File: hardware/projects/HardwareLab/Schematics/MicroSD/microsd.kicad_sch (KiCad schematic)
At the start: 3 parts, among them J1 Conn_01x03

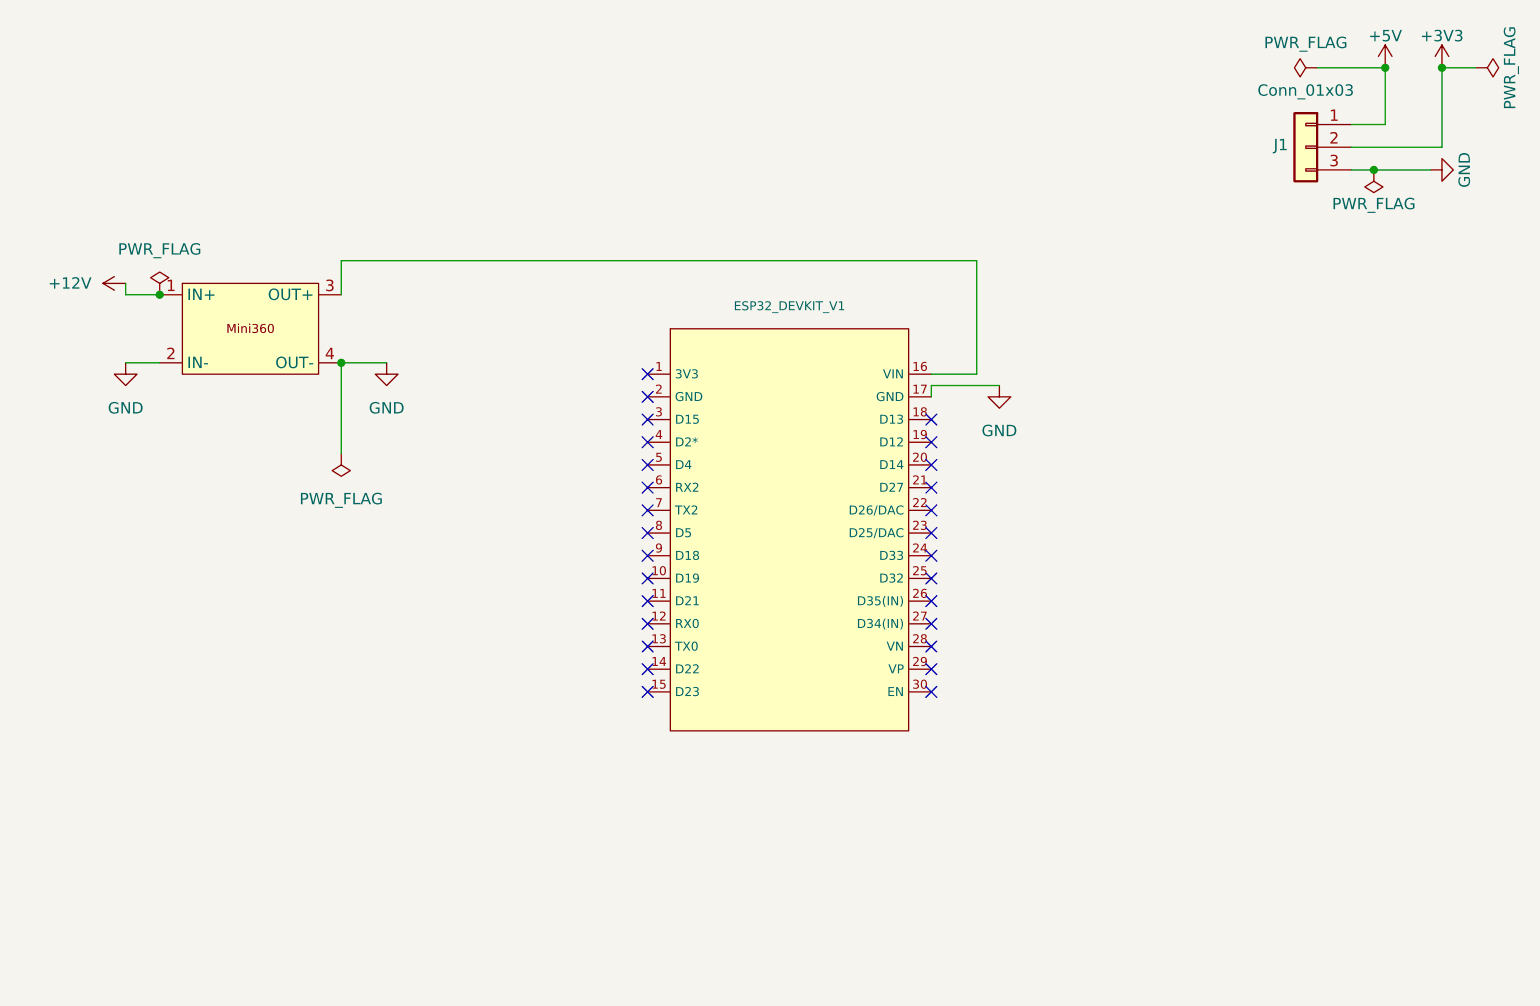
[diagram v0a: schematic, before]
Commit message: Evolução de bibliotecas de componentes criada.
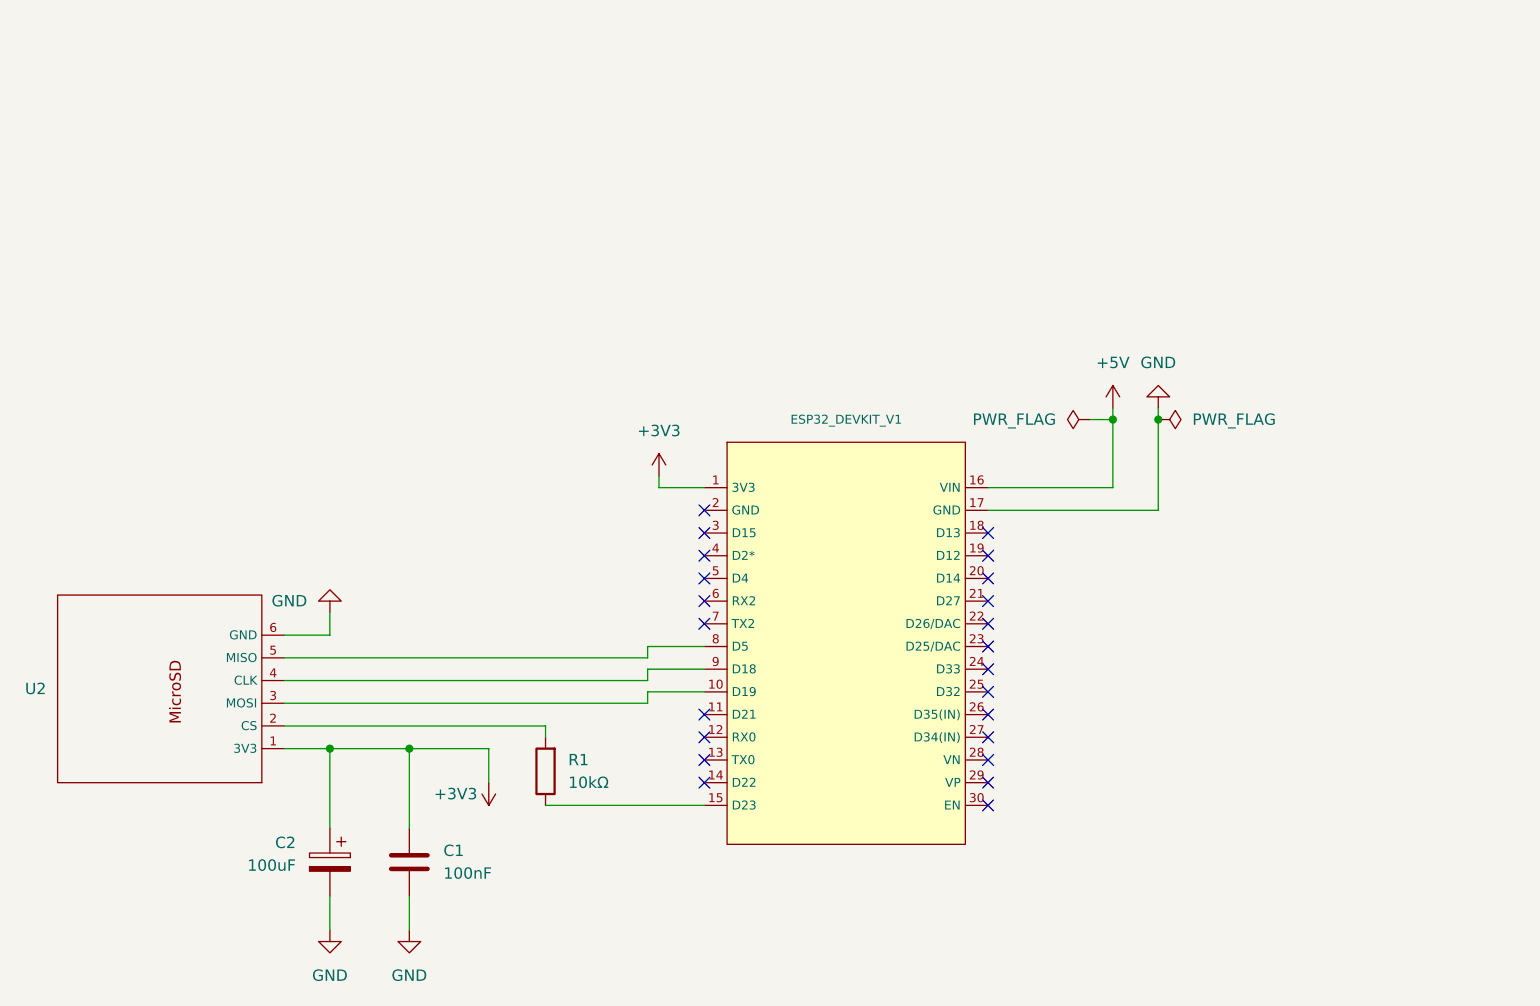
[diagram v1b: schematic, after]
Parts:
- removed J1: Conn_01x03, symbol Connector_Generic:Conn_01x03
- removed PS1: (no value), TechBaseLab:Mini360_Buck_Converter, symbol TechBaseLab:Mini360_Buck_Converter
- added C1: 100nF, symbol Device:C
- added C2: 100uF, symbol Device:C_Polarized
- added R1: 10kΩ, symbol Device:R
- added U2: (no value), TechBaseLab:MicroSD_Module_Mini_21x18mm_1x6_P2.54mm, symbol TechBaseLab:MicroSD_Module_Mini
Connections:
- net +3V3: now also ESP32_DEVKIT_V1.1 (3V3), C1.1, C2.1, U2.1 (3V3)
- net +5V: now also ESP32_DEVKIT_V1.16 (VIN)
- net GND: now also C1.2, C2.2, U2.6 (GND)
- net at ESP32_DEVKIT_V1.10 (D19): now also U2.3 (MOSI)
- net at ESP32_DEVKIT_V1.15 (D23): now also R1.1
- net at ESP32_DEVKIT_V1.8 (D5): now also U2.5 (MISO)
- net at ESP32_DEVKIT_V1.9 (D18): now also U2.4 (CLK)
- new net: R1.2, U2.2 (CS)
- no-connect marks 28 -> 23
